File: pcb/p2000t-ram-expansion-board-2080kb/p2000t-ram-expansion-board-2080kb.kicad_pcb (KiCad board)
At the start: 2 copper layers, 108.6 x 66.8 mm, 30 parts, among them J1 EXPANSION BOARD, J2 POWER, J3 TERMINAL, U1 74HC04, U10 AS6C4008-55PCN, U11 AS6C4008-55PCN, U12 74HC138, U13 74HC74, U2 AS6C4008-55PCN, U3 74HC00, U4 CY62256-70PC, U5 74HC688, U6 74HC32, U7 74HC273, U8 74HC245, U9 AS6C4008-55PCN

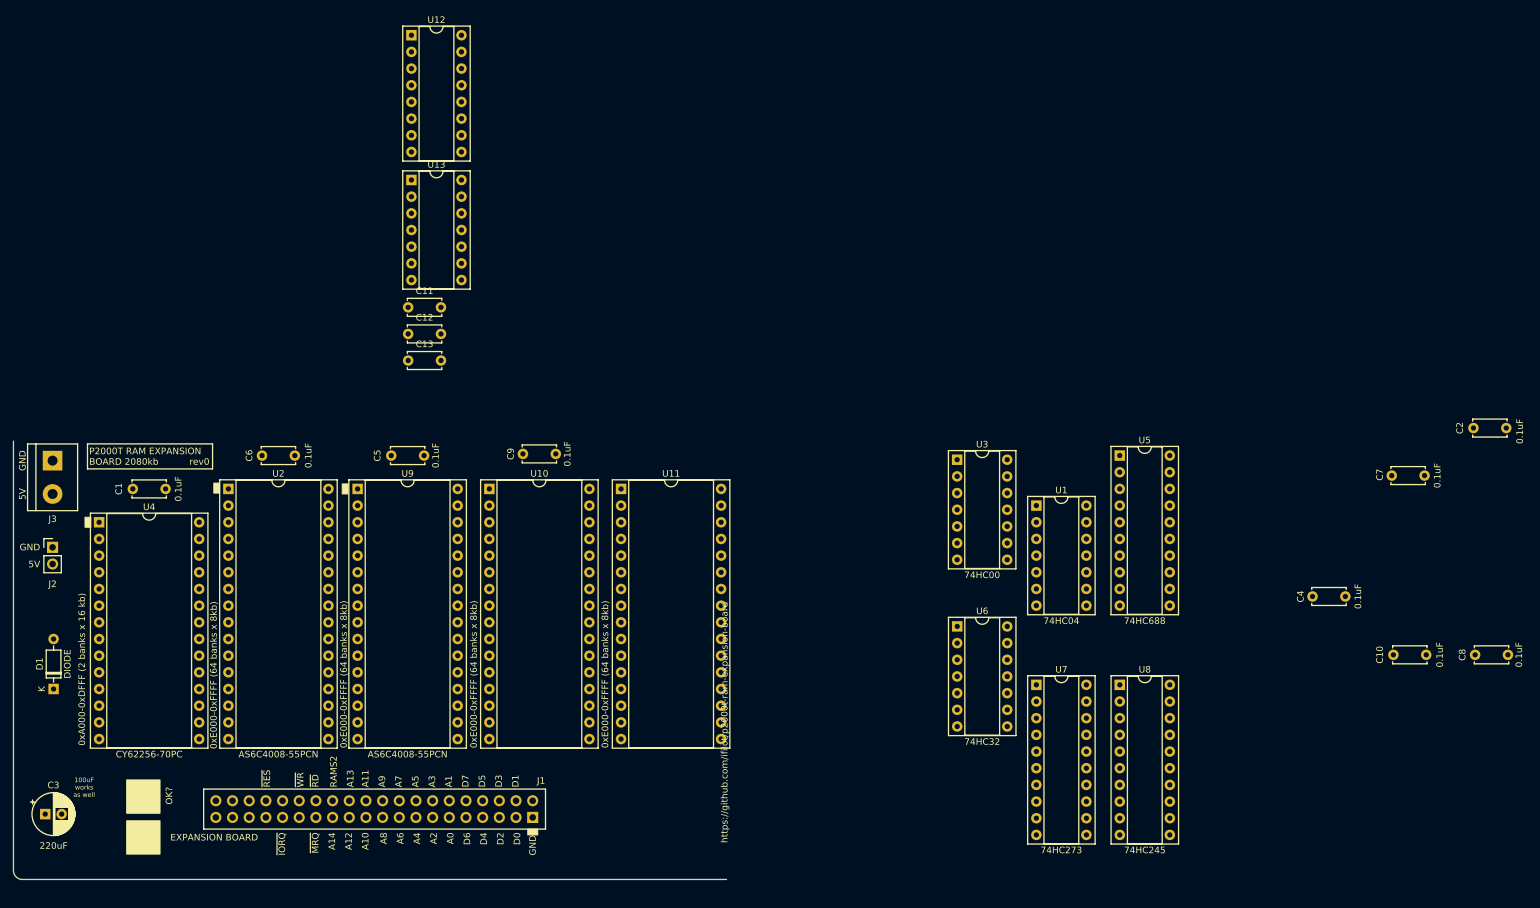
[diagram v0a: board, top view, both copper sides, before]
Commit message: Adding gerbers
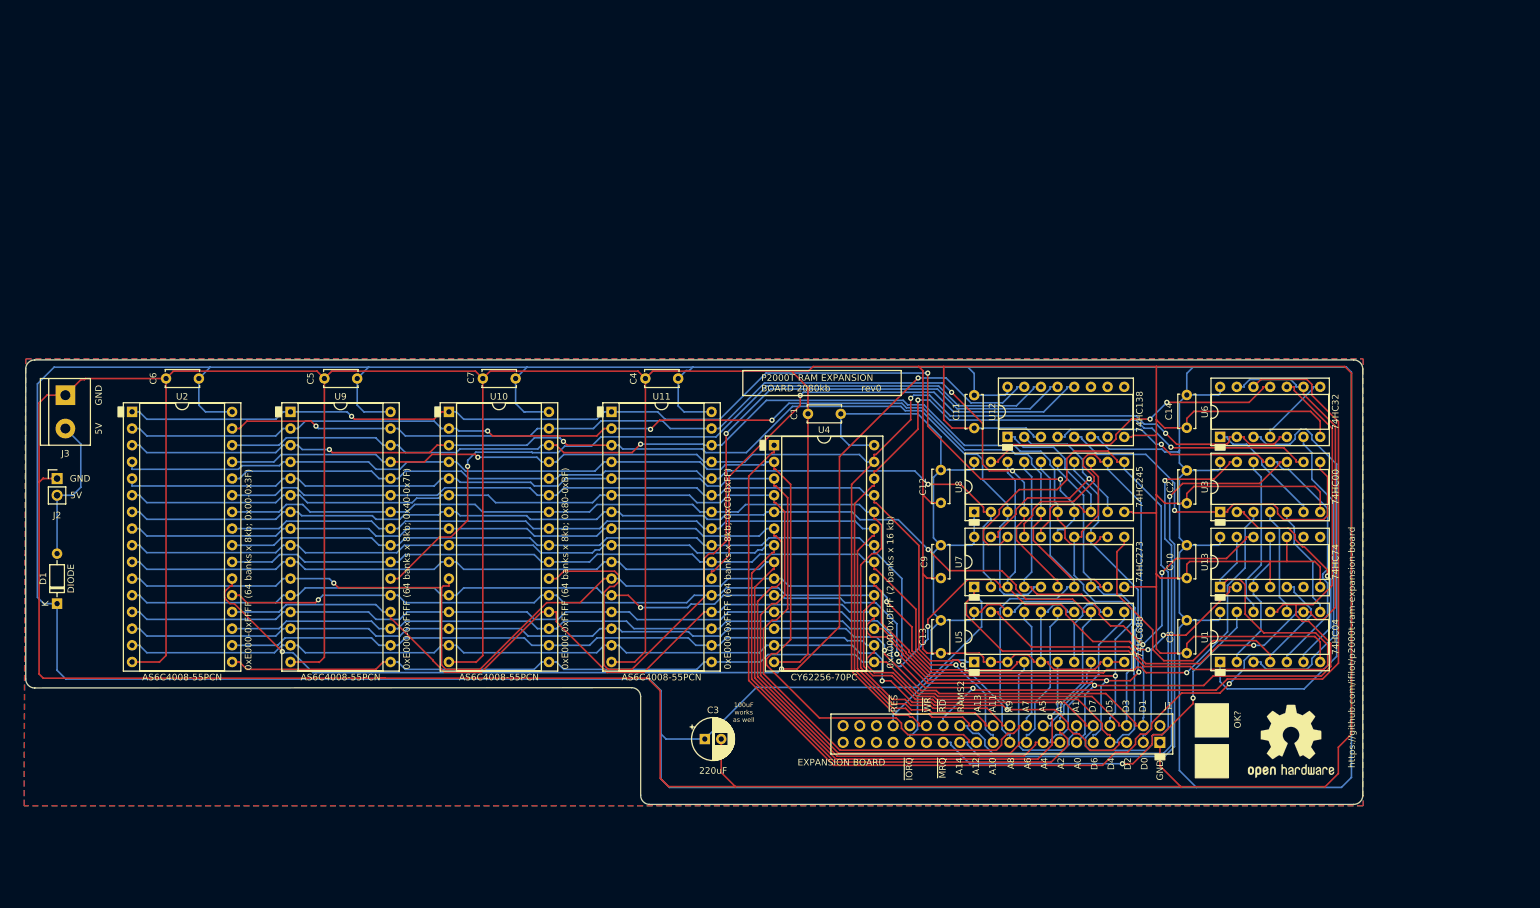
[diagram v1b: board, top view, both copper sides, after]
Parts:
- added C14: 0.1uF, Capacitor_THT:C_Disc_D5.0mm_W2.5mm_P5.00mm, F.Cu at (212.9, 74.3)
- added REF**: OSHW-Logo2_14.6x12mm_SilkScreen, Symbol:OSHW-Logo2_14.6x12mm_SilkScreen, F.Cu at (228.8, 127.1)
- moved C7 139.2 mm to (110.7, 71.8)
- moved U13 137.9 mm to (218.0, 103.6), turned to 90 degrees
- moved U12 109.5 mm to (185.6, 80.7), turned to 90 degrees
- moved C4 106.9 mm to (135.4, 71.8)
- moved C1 103.5 mm to (160.2, 77.2)
- moved U4 103.5 mm to (150.1, 82.0)
- moved C3 101.1 mm to (139.5, 126.7)
- moved J1 96.2 mm to (208.8, 127.3)
- moved C13 90.3 mm to (175.5, 108.7), turned to -90 degrees
- moved C11 87.3 mm to (180.5, 74.4), turned to -90 degrees
- moved C12 83.7 mm to (175.5, 85.8), turned to -90 degrees
- moved C9 60.3 mm to (175.5, 97.2), turned to -90 degrees
- moved U6 49.4 mm to (218.0, 80.7), turned to 90 degrees
- moved C8 49.2 mm to (212.9, 108.7), turned to -90 degrees
- moved C2 49.1 mm to (212.9, 85.8), turned to -90 degrees
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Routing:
- net GND: track 0.00 -> 1093.0 mm
- net +5V: track 0.00 -> 855.0 mm
- net A0: track 0.00 -> 263.6 mm, vias 0 -> 3
- net ~{RD}: track 0.00 -> 253.2 mm, vias 0 -> 2
- net D7: track 0.00 -> 249.7 mm, vias 0 -> 1
- net D1: track 0.00 -> 248.1 mm, vias 0 -> 3
- net D6: track 0.00 -> 234.6 mm, vias 0 -> 2
- net D0: track 0.00 -> 229.4 mm, vias 0 -> 3
- net ~{WR}: track 0.00 -> 224.8 mm, vias 0 -> 3
- net D2: track 0.00 -> 215.3 mm, vias 0 -> 2
- net A4: track 0.00 -> 202.4 mm
- net A7: track 0.00 -> 200.1 mm
- net A6: track 0.00 -> 200.1 mm
- net D4: track 0.00 -> 199.2 mm
- net A3: track 0.00 -> 193.3 mm
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- added copper zone on B.Cu, net +5V
- added copper zone on F.Cu, net GND
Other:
- board size 108.6 x 66.8 mm -> 203.7 x 67.7 mm
- board text added: "0xE000-0xFFFF (64 banks x 8kb; 0x00-0x3F)"
- board text added: "0xE000-0xFFFF (64 banks x 8kb; 0x40-0x7F)"
- board text added: "0xE000-0xFFFF (64 banks x 8kb; 0x80-0xBF)"
- board text added: "0xE000-0xFFFF (64 banks x 8kb; 0xC0-0xFF)"
- board text removed: "0xE000-0xFFFF (64 banks x 8kb)"
